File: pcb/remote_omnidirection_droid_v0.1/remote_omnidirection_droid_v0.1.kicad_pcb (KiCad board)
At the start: 2 copper layers, 120 x 103.9 mm, 76 parts, among them J1 USB_C_Receptacle_USB2.0, J2 Conn_01x04, J3 BATT_CONNECT, J4 Conn_01x04, J5 Conn_01x04, M1 Motor_DC_ALT, M2 Motor_DC_ALT, M3 Motor_DC_ALT, Q1 BC846BS, SW1 SW_SPST, SW2 SW_SPST, SW3 SW_SPDT, U1 AZ1117-3.3, U2 AZ1117-5.0, U3 USBLC6-2SC6, U4 ESP32-S3-WROOM-2-N32R8V, U5 PCA9685PW, U6 BNO055, U7 PCA9306D, Y1 32.768kHz

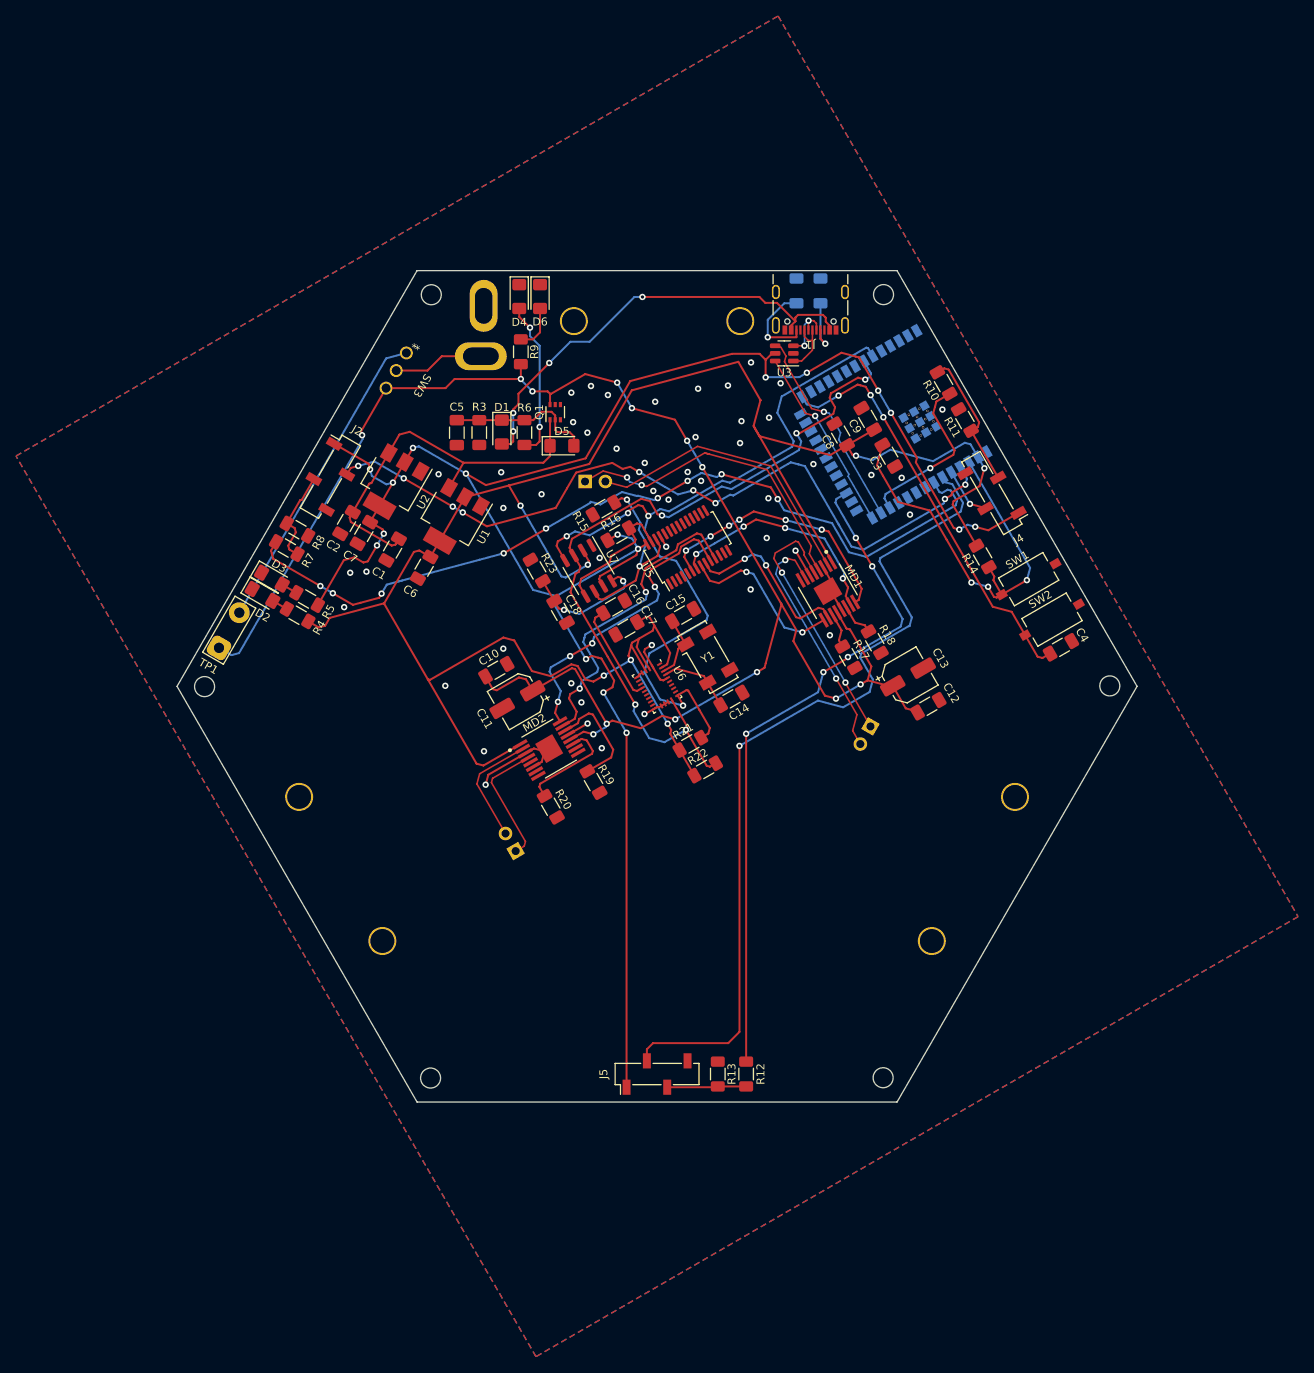
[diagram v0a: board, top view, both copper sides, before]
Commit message: near finalized v0.1
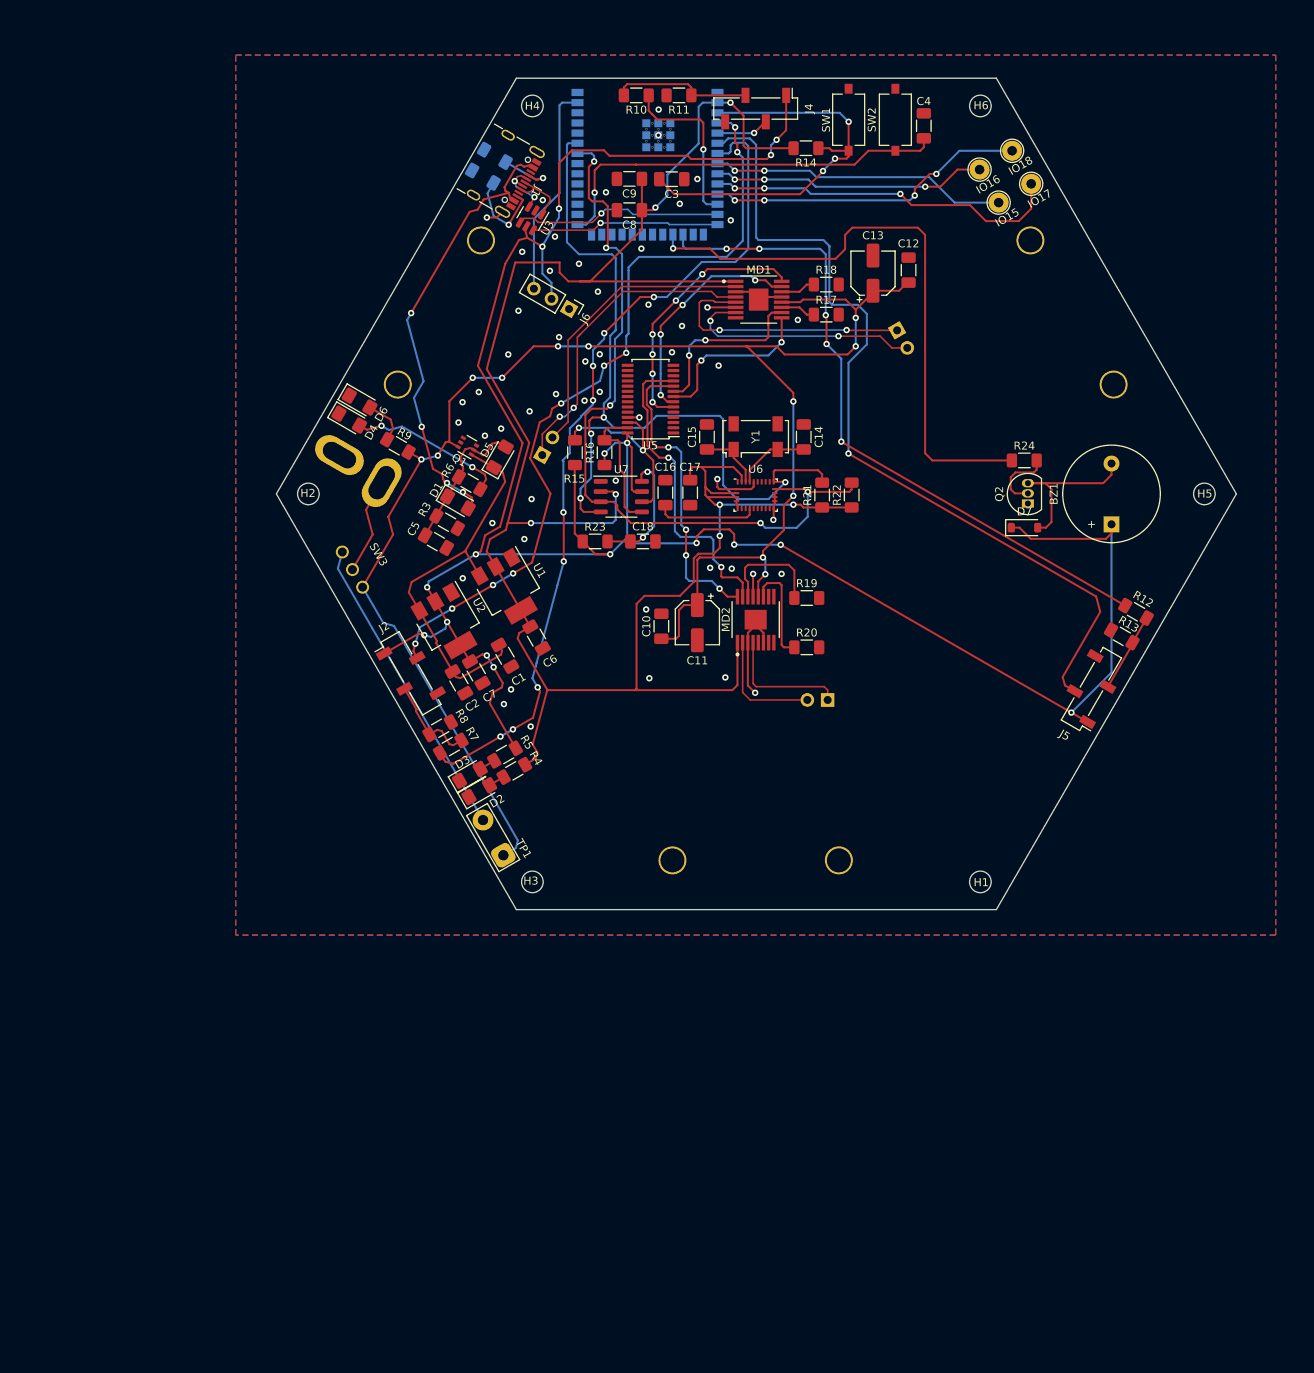
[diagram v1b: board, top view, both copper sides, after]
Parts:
- added BZ1: Buzzer, Buzzer_Beeper:Buzzer_12x9.5RM7.6, F.Cu at (159.7, 92.0)
- added D7: 1N4148W, Diode_SMD:D_SOD-123, F.Cu at (148.9, 92.5)
- added IO15: TestPoint, TestPoint:TestPoint_THTPad_D2.5mm_Drill1.2mm, F.Cu at (145.6, 51.8)
- added IO16: TestPoint, TestPoint:TestPoint_THTPad_D2.5mm_Drill1.2mm, F.Cu at (143.2, 47.7)
- added IO17: TestPoint, TestPoint:TestPoint_THTPad_D2.5mm_Drill1.2mm, F.Cu at (149.7, 49.5)
- added IO18: TestPoint, TestPoint:TestPoint_THTPad_D2.5mm_Drill1.2mm, F.Cu at (147.3, 45.4)
- added J6: Conn_01x03, Connector_PinHeader_2.54mm:PinHeader_1x03_P2.54mm_Vertical, F.Cu at (91.9, 65.1)
- added Q2: 2N2219, Package_TO_SOT_THT:TO-92L_Inline, F.Cu at (149.3, 89.4)
- added R24: 180, Resistor_SMD:R_1206_3216Metric_Pad1.30x1.75mm_HandSolder, F.Cu at (148.8, 84.1)
- H1, H2, H3, H4, H5, H6: footprint MountingHole:MountingHole_2.5mm -> MountingHole:MountingHole_2.7mm_M2.5
- moved H4 129.1 mm to (87.3, 39.8), turned to 0 degrees
- moved H5 121.2 mm to (171.3, 88.2), turned to 0 degrees
- moved H6 121.1 mm to (143.3, 39.8), turned to 0 degrees
- moved H1 100.5 mm to (143.3, 136.7), turned to 0 degrees
- moved H3 76.2 mm to (87.3, 136.7), turned to 0 degrees
- moved H2 76.1 mm to (59.3, 88.2), turned to 0 degrees
- moved R12 75.6 mm to (162.8, 103.0), turned to -30 degrees
- moved R13 74.5 mm to (161.0, 106.1), turned to 150 degrees
- moved J5 72.6 mm to (157.2, 112.6), turned to 150 degrees
- moved C4 67.4 mm to (136.3, 42.2), turned to 90 degrees
- moved SW2 65.5 mm to (132.7, 41.5), turned to -90 degrees
- moved SW1 61.7 mm to (126.9, 41.5), turned to -90 degrees
- moved M2 60.4 mm to (145.8, 70.8), turned to -60 degrees
- moved J4 56.4 mm to (115.3, 40.1), turned to -90 degrees
- moved R14 55.6 mm to (121.5, 45.0), turned to 180 degrees
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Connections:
- MD1 pad 8: /nFAULT -> unconnected-(MD1-nFAULT-Pad8)
- MD2 pad 8: /nFAULT1 -> unconnected-(MD2-nFAULT-Pad8)
- U4 pad 10: unconnected-(U4-IO17-Pad10) -> /IO17
- U4 pad 11: unconnected-(U4-IO18-Pad11) -> /IO18
- U4 pad 18: unconnected-(U4-IO10-Pad18) -> /BUZZER
- U4 pad 39: unconnected-(U4-IO1-Pad39) -> /NeoPixel
- U4 pad 8: unconnected-(U4-IO15-Pad8) -> /IO15
- U4 pad 9: unconnected-(U4-IO16-Pad9) -> /IO16
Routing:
- net /BUZZER: track 0.00 -> 75.4 mm, vias 0 -> 1
- net +5V: track 249.8 -> 312.0 mm
- net /IO17: track 0.00 -> 44.9 mm, vias 0 -> 3
- net /IO18: track 0.00 -> 40.2 mm, vias 0 -> 4
- net /IO15: track 0.00 -> 37.2 mm, vias 0 -> 2
- net /IO16: track 0.00 -> 34.3 mm, vias 0 -> 3
- net /NeoPixel: track 0.00 -> 26.6 mm
- net Net-(BZ1-+): track 0.00 -> 21.7 mm
- net Net-(Q2-B): track 0.00 -> 8.66 mm
- net GND: track 37.4 -> 39.7 mm, vias 49 -> 53
- net +3V3: track 267.2 -> 269.3 mm
- net Net-(SW3-A): track 39.3 -> 38.4 mm
- net Net-(J3-Pin_1): track 11.3 -> 12.2 mm
- net /NESD_D+: track 7.48 -> 8.10 mm
- net +BATT: track 206.1 -> 206.3 mm, vias 13 -> 12
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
